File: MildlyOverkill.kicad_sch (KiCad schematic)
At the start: 94 parts, among them J1 USB_C_Receptacle_USB2.0_16P, J2 Screw_Terminal_01x02, J3 Motors, J4 IO, J5 Conn_01x04_Pin, J6 Conn_01x04_MountingPin, J8 RJ45_Wuerth_7499010211A, J9 Analog, M1 Fan_4pin, U1 ESP32-S3-WROOM-1, U2 MCP3208, U3 LD1117S33TR_SOT223, U5 USBLC6-2P6, U6 TPS62932, U7 W5500, Y1 3134250001

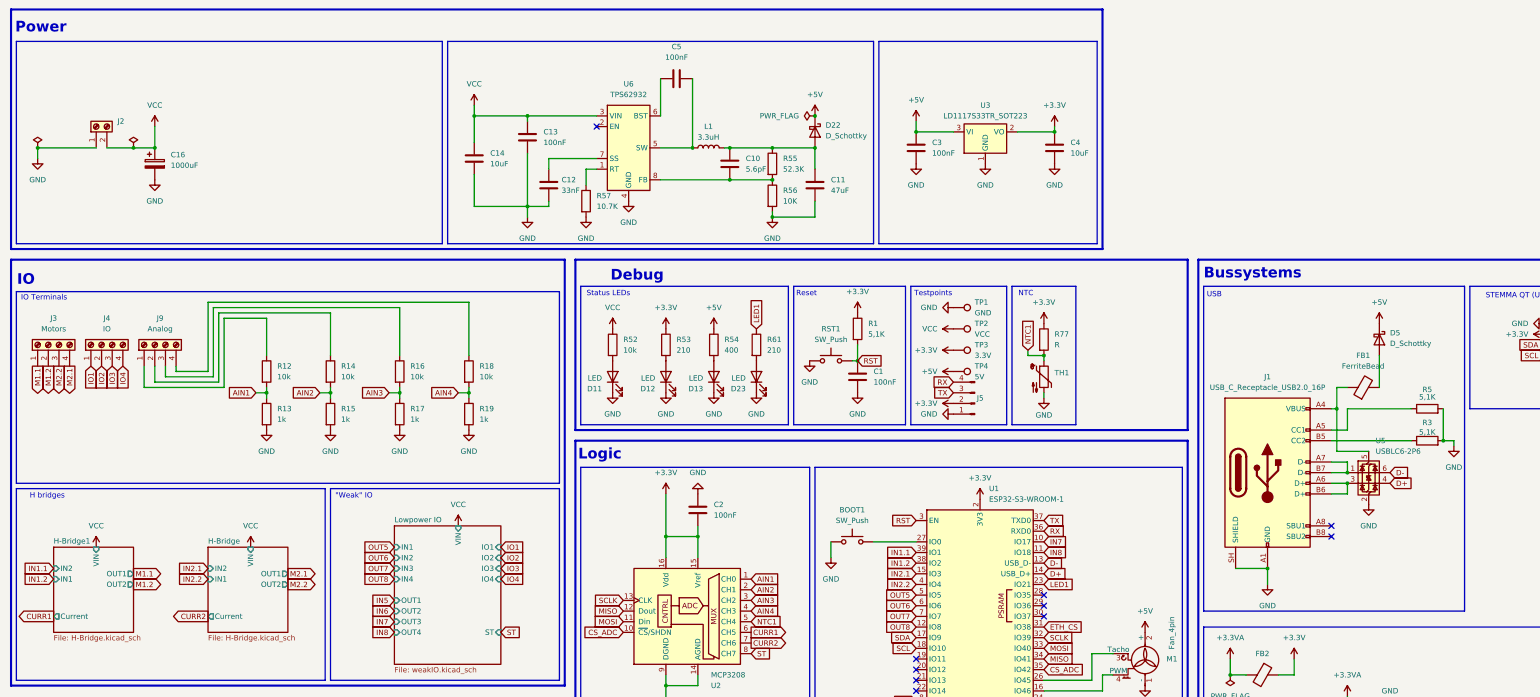
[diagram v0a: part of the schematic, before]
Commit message: H-Bridges are done i guess
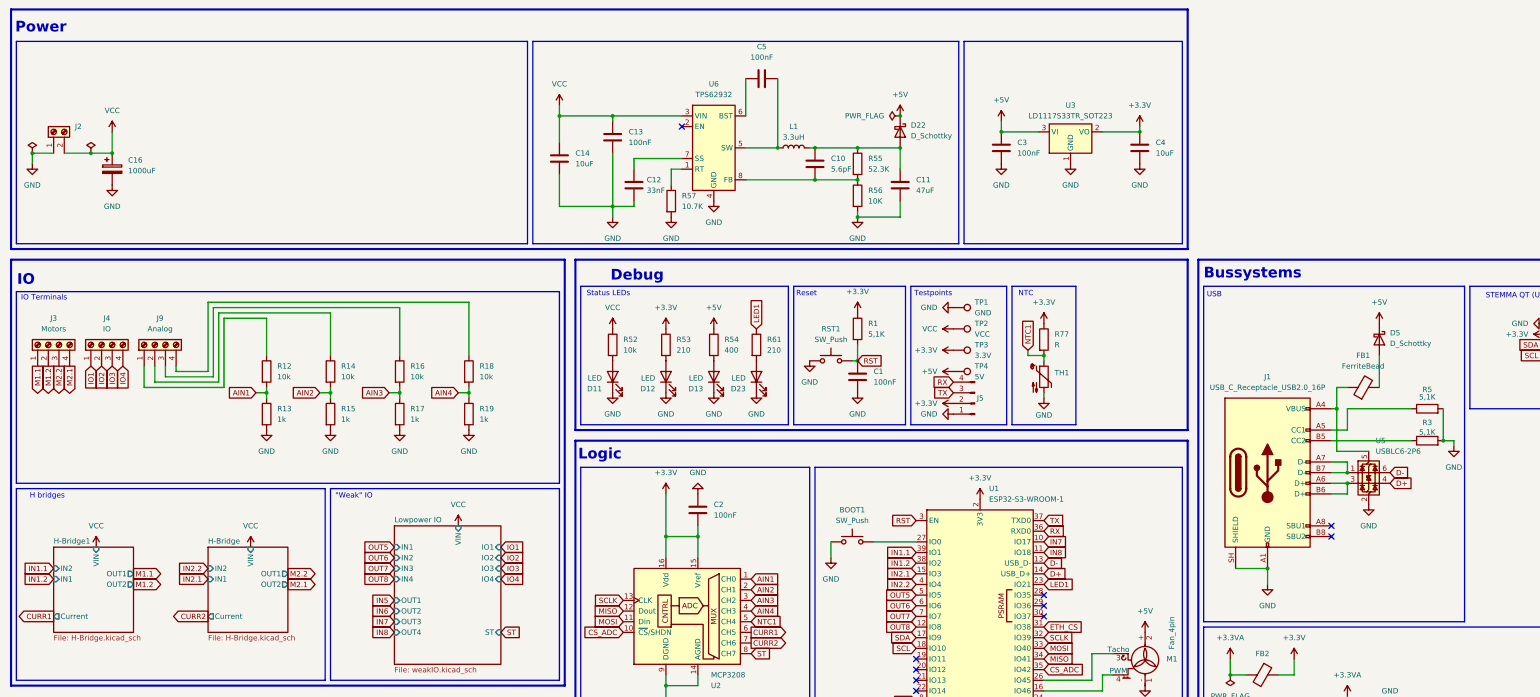
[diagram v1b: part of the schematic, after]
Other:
- moved on the sheet: C10, C11, C12, C13, C14, C16, C3, C4, C5, D22, J2, L1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

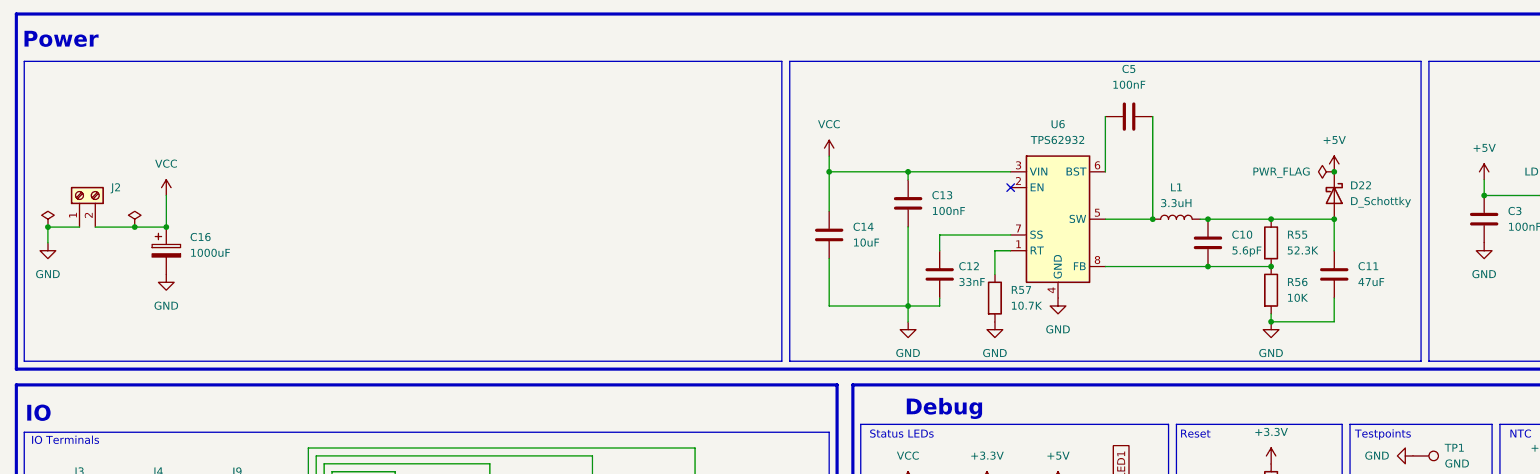
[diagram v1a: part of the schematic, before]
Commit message: Power stage almost done
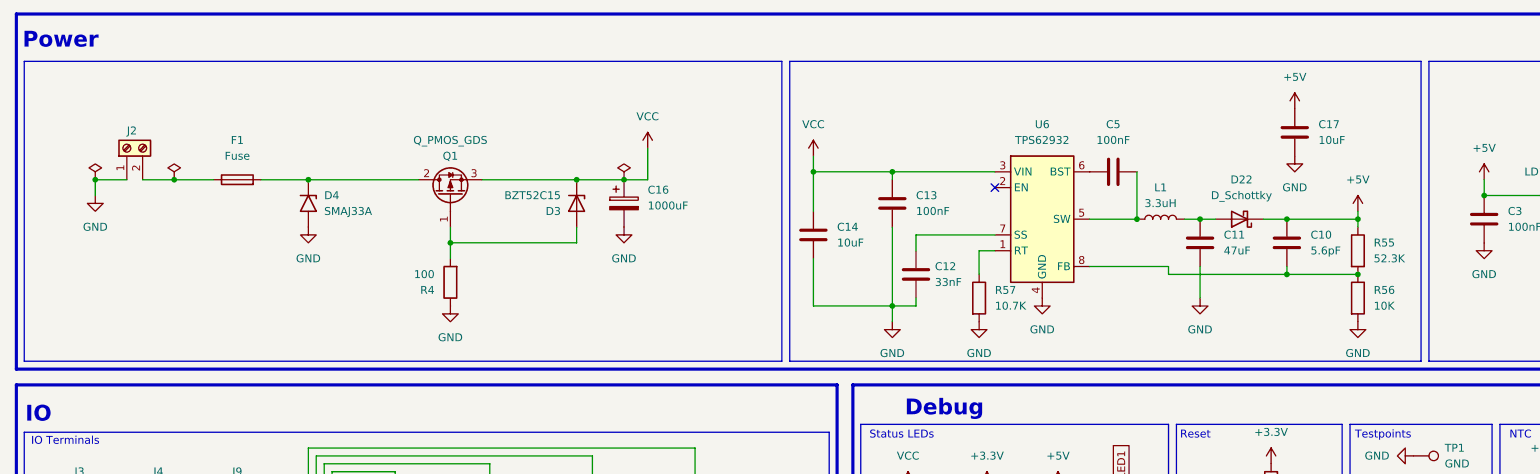
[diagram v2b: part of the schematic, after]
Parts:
- added C17: 10uF, Capacitor_SMD:C_0603_1608Metric, symbol Device:C
- added D3: BZT52C15, Diode_SMD:D_0805_2012Metric, symbol Device:D_Zener
- added D4: SMAJ33A, Diode_SMD:D_SMA, symbol Diode:SMAJ33A
- added F1: Fuse, Fuse:Fuseholder_Blade_Mini_Keystone_3568, symbol Device:Fuse
- added Q1: Q_PMOS_GDS, Package_TO_SOT_SMD:TO-252-2, symbol Transistor_FET:Q_PMOS_GDS
- added R4: 100, Resistor_SMD:R_0805_2012Metric, symbol Device:R
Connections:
- net +5V: now also C10.2, R55.1, C17.2
- net GND: now also C17.1, D4.2 (A2), R4.1
- net VCC: now also D3.1 (K), Q1.3 (S); no longer J2.2 (Pin_2)
- net at C11.2, D22.2 (A), L1.2: no longer C10.2, R55.1
- new net: D4.1 (A1), F1.2, Q1.2 (D)
- new net: F1.1, J2.2 (Pin_2)
- new net: D3.2 (A), Q1.1 (G), R4.2
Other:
- moved on the sheet: C10, C11, C12, C13, C14, C16, C5, D22, J2, L1, R55, R56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

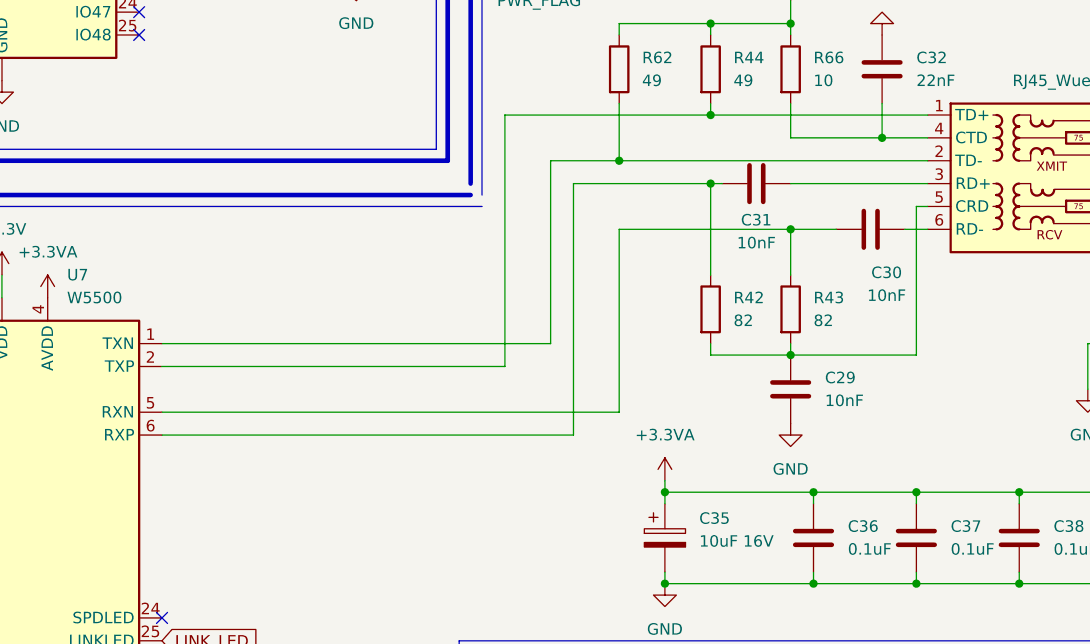
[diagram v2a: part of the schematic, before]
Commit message: Insane amounts of routing and Ethernet ist basicaly done.
DRC is going to be fun for future me...
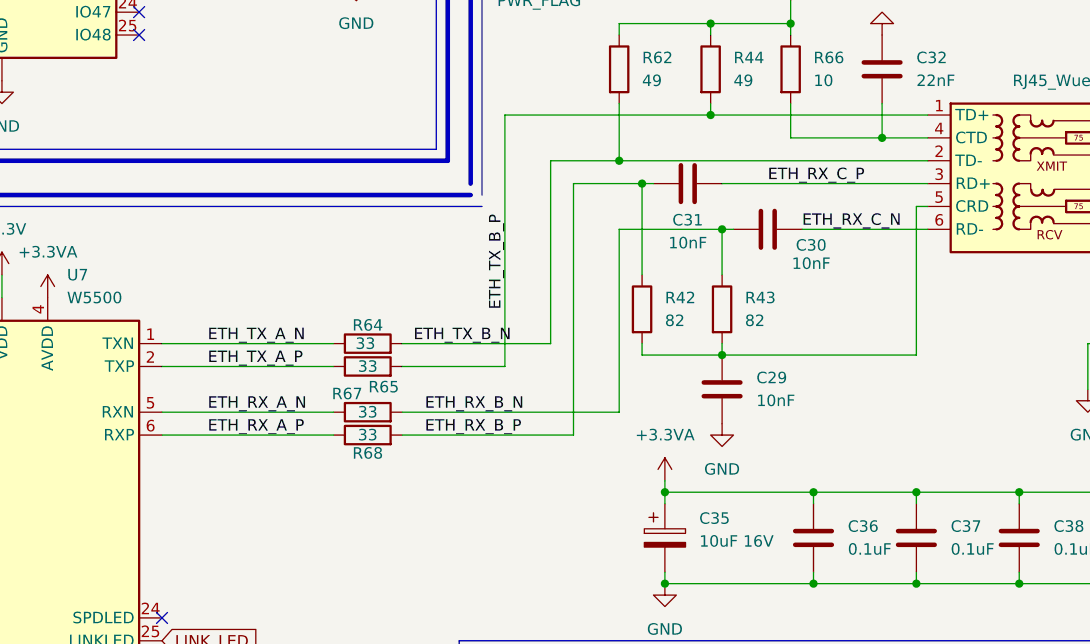
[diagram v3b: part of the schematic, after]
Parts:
- added R64, R65, R67, R68: 33, Resistor_SMD:R_0603_1608Metric, symbol Device:R
- C29, C30, C31, C32: footprint Capacitor_SMD:C_0805_2012Metric -> Capacitor_SMD:C_0603_1608Metric
- R42, R43, R44, R62, R66: footprint Resistor_SMD:R_0805_2012Metric -> Resistor_SMD:R_0603_1608Metric
- R74: footprint Capacitor_SMD:C_0603_1608Metric_Pad1.08x0.95mm_HandSolder -> Resistor_SMD:R_0805_2012Metric_Pad1.20x1.40mm_HandSolder
- Y1: footprint Crystal:Crystal_SMD_3225-4Pin_3.2x2.5mm_HandSoldering -> Crystal:Crystal_SMD_3225-4Pin_3.2x2.5mm
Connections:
- net ETH_RX_B_N: now reaches C30.1, R43.1
- net ETH_RX_B_N: now also R67.2; no longer U7.5 (RXN)
- net ETH_RX_C_N: now reaches C30.2, J8.6 (RD-)
- net ETH_TX_B_P: now reaches J8.1 (TD+), R44.2
- net ETH_TX_B_P: now also R65.2; no longer U7.2 (TXP)
- net ETH_TX_B_N: now reaches J8.2 (TD-), R62.2
- net ETH_TX_B_N: now also R64.2; no longer U7.1 (TXN)
- net ETH_RX_B_P: now reaches C31.1, R42.1
- net ETH_RX_B_P: now also R68.2; no longer U7.6 (RXP)
- net ETH_RX_C_P: now reaches C31.2, J8.3 (RD+)
- new net ETH_RX_A_N: R67.1, U7.5 (RXN)
- new net ETH_RX_A_P: R68.1, U7.6 (RXP)
- new net ETH_TX_A_N: R64.1, U7.1 (TXN)
- new net ETH_TX_A_P: R65.1, U7.2 (TXP)
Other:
- moved on the sheet: C29, C30, C31, R42, R43
